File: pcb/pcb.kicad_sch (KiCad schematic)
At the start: 66 parts, among them IC1 W25Q16JVUXIQ, IC2 RP2040, IC3 AD8403ARUZ1-REEL, IC4 DS4432U+, IC5 XC6222D331MR-G, J1 USB_C_Receptacle, K1 G3VM-31WR_TR05_, Y2 ABM10AIG-12.000MHZ-2Z-T

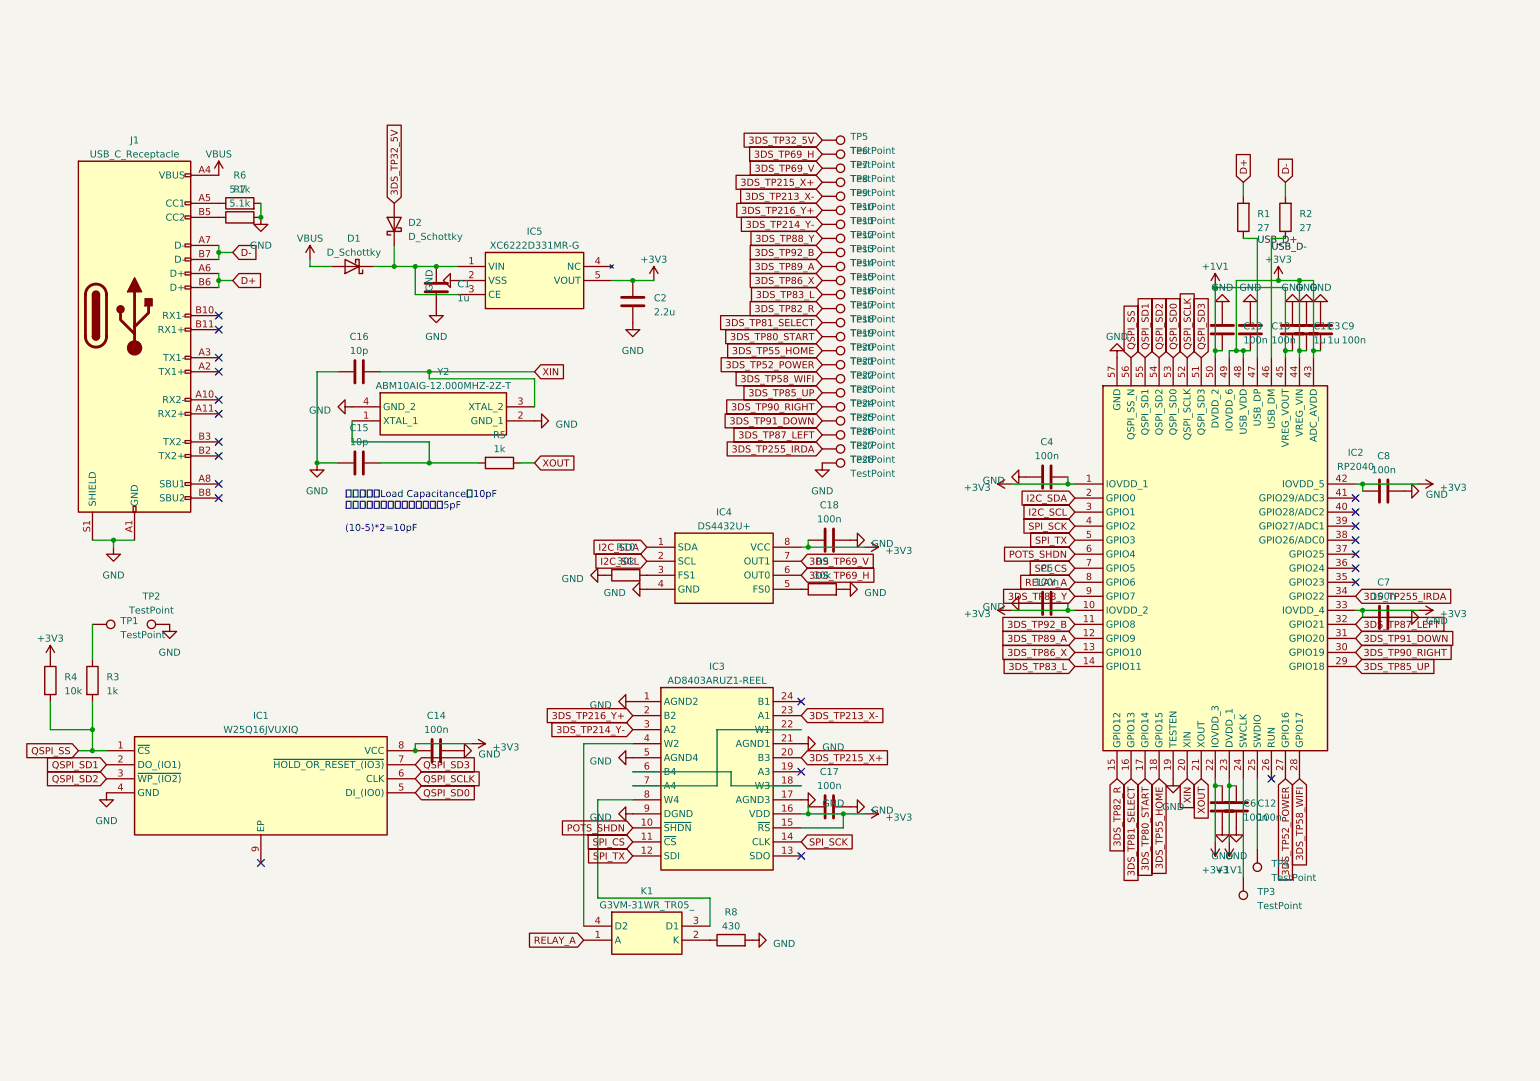
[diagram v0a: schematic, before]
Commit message: Update pcb
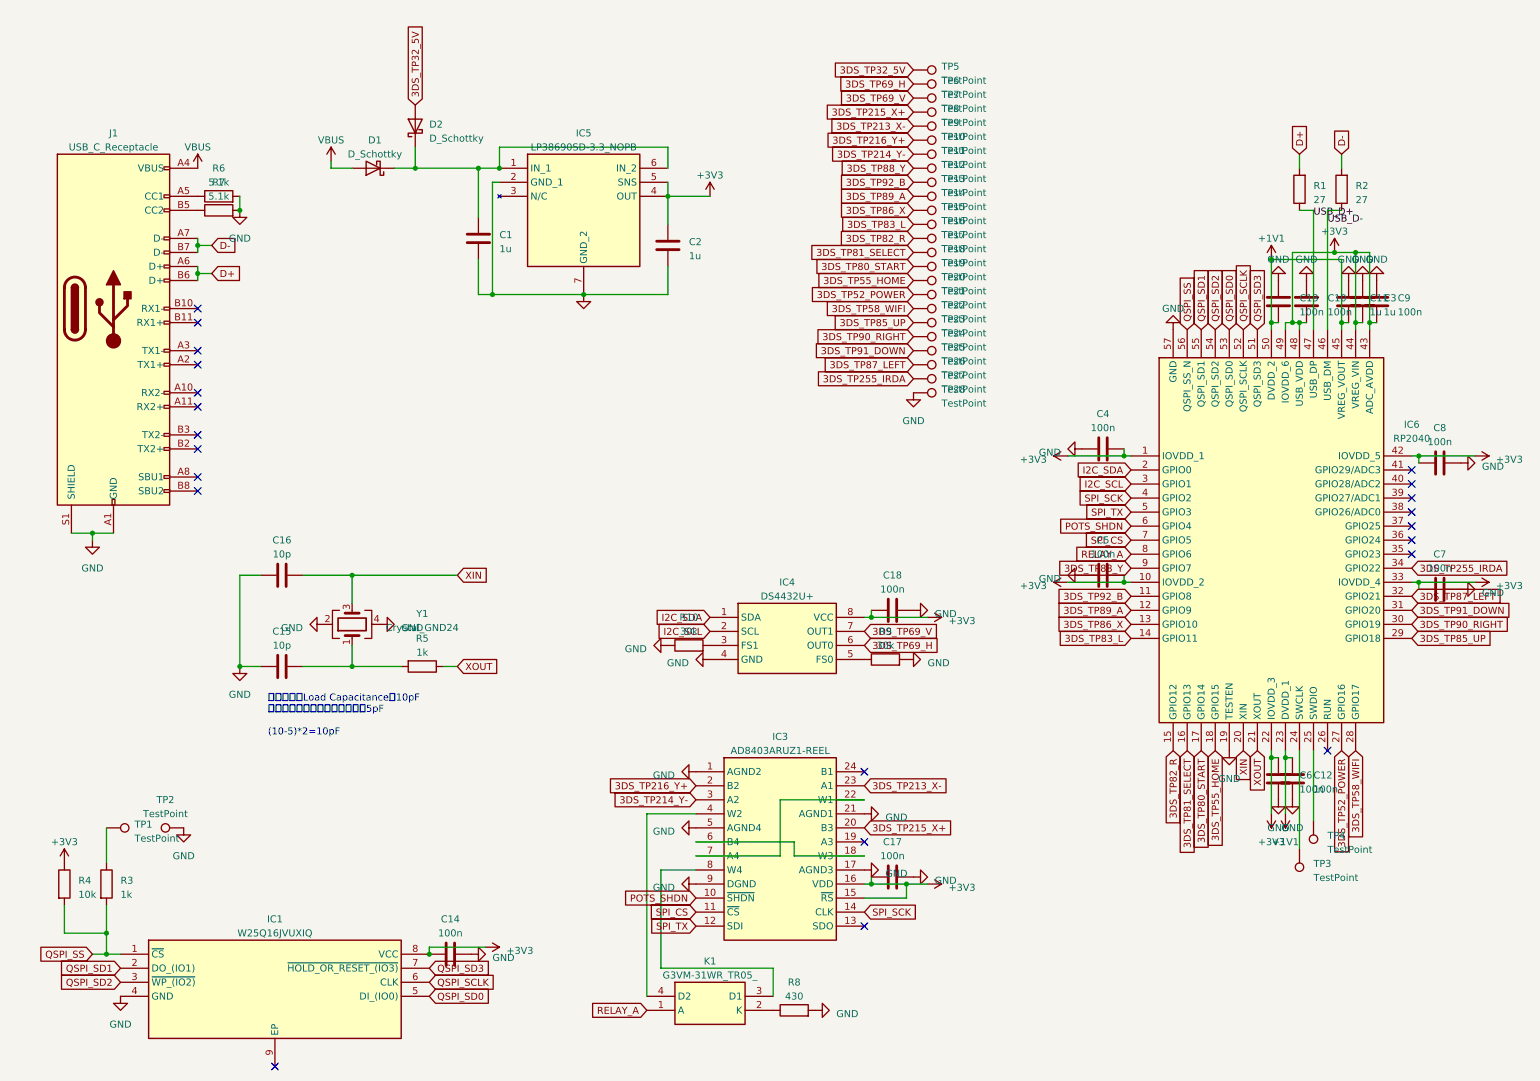
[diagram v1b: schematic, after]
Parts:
- removed IC2: RP2040, RP2040:QFN40P700X700X90-57N-D, symbol RP2040:RP2040
- removed IC5: XC6222D331MR-G, XC6222D331MR-G:SOT95P280X130-5N, symbol XC6222D331MR-G:XC6222D331MR-G
- removed Y2: ABM10AIG-12.000MHZ-2Z-T, ABM10AIG-12.000MHZ-2Z-T:ABM10AIG, symbol ABM10AIG-12_000MHZ-2Z-T:ABM10AIG-12.000MHZ-2Z-T
- added IC5: LP38690SD-3.3_NOPB, LP38690SD-3.3_NOPB:SON95P300X300X80-7N, symbol LP38690SD-3_3_NOPB:LP38690SD-3.3_NOPB
- added IC6: RP2040, RP2040:QFN40P700X700X90-57N-D, symbol RP2040:RP2040
- added Y1: Crystal_GND24, Crystal:Crystal_SMD_2520-4Pin_2.5x2.0mm, symbol Device:Crystal_GND24
- C1, C11, C3: footprint Capacitor_SMD:C_0201_0603Metric -> Capacitor_SMD:C_0402_1005Metric; LCSC C610030 -> C412453
- C10, C12, C13, C14, C17, C18, C4, C5, C6, C7, C8, C9: footprint Capacitor_SMD:C_0201_0603Metric -> Capacitor_SMD:C_0402_1005Metric; LCSC C5259862 -> C394158
- C15, C16: footprint Capacitor_SMD:C_0201_0603Metric -> Capacitor_SMD:C_0402_1005Metric; LCSC C396694 -> C161495
- C2: value 2.2u -> 1u; footprint Capacitor_SMD:C_0201_0603Metric -> Capacitor_SMD:C_0402_1005Metric; LCSC C5240383 -> C412453
- IC1: LCSC C2843335 -> (none)
- IC3: LCSC C652779 -> (none)
- IC4: LCSC C2679620 -> (none)
- R1, R2: footprint Resistor_SMD:R_0201_0603Metric -> Resistor_SMD:R_0402_1005Metric; LCSC C2484262 -> C102938
- R10, R9: footprint Resistor_SMD:R_0201_0603Metric -> Resistor_SMD:R_0402_1005Metric; LCSC C2991673 -> C144716
- R3, R5: footprint Resistor_SMD:R_0201_0603Metric -> Resistor_SMD:R_0402_1005Metric; LCSC C162776 -> C705665
- R4: footprint Resistor_SMD:R_0201_0603Metric -> Resistor_SMD:R_0402_1005Metric; LCSC C253350 -> C2991755
- R6, R7: footprint Resistor_SMD:R_0201_0603Metric -> Resistor_SMD:R_0402_1005Metric; LCSC C100142 -> C138073
- R8: footprint Resistor_SMD:R_0201_0603Metric -> Resistor_SMD:R_0402_1005Metric; LCSC C850675 -> C163462
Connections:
- net +1V1: now also IC6.23 (DVDD_1), IC6.45 (VREG_VOUT), IC6.50 (DVDD_2)
- net +3V3: now also IC5.4 (OUT), IC5.5 (SNS), IC6.1 (IOVDD_1), IC6.10 (IOVDD_2), IC6.22 (IOVDD_3), IC6.33 (IOVDD_4), IC6.42 (IOVDD_5), IC6.43 (ADC_AVDD), IC6.44 (VREG_VIN), IC6.48 (USB_VDD), IC6.49 (IOVDD_6)
- net 3DS_TP255_IRDA: now also IC6.34 (GPIO22)
- net 3DS_TP52_POWER: now also IC6.27 (GPIO16)
- net 3DS_TP55_HOME: now also IC6.18 (GPIO15)
- net 3DS_TP58_WIFI: now also IC6.28 (GPIO17)
- net 3DS_TP80_START: now also IC6.17 (GPIO14)
- net 3DS_TP81_SELECT: now also IC6.16 (GPIO13)
- net 3DS_TP82_R: now also IC6.15 (GPIO12)
- net 3DS_TP83_L: now also IC6.14 (GPIO11)
- net 3DS_TP85_UP: now also IC6.29 (GPIO18)
- net 3DS_TP86_X: now also IC6.13 (GPIO10)
- net 3DS_TP87_LEFT: now also IC6.32 (GPIO21)
- net 3DS_TP88_Y: now also IC6.9 (GPIO7)
- net 3DS_TP89_A: now also IC6.12 (GPIO9)
- net 3DS_TP90_RIGHT: now also IC6.30 (GPIO19)
- net 3DS_TP91_DOWN: now also IC6.31 (GPIO20)
- net 3DS_TP92_B: now also IC6.11 (GPIO8)
- net GND: now also IC5.2 (GND_1), IC5.7 (GND_2), IC6.19 (TESTEN), IC6.57 (GND), Y1.2, Y1.4
- net I2C_SCL: now also IC6.3 (GPIO1)
- net I2C_SDA: now also IC6.2 (GPIO0)
- net POTS_SHDN: now also IC6.6 (GPIO4)
- net QSPI_SCLK: now also IC6.52 (QSPI_SCLK)
- net QSPI_SD0: now also IC6.53 (QSPI_SD0)
- net QSPI_SD1: now also IC6.55 (QSPI_SD1)
- net QSPI_SD2: now also IC6.54 (QSPI_SD2)
- net QSPI_SD3: now also IC6.51 (QSPI_SD3)
- net QSPI_SS: now also IC6.56 (QSPI_SS_N)
- net RELAY_A: now also IC6.8 (GPIO6)
- net SPI_CS: now also IC6.7 (GPIO5)
- net SPI_SCK: now also IC6.4 (GPIO2)
- net SPI_TX: now also IC6.5 (GPIO3)
- net USB_D+: now also IC6.47 (USB_DP)
- net USB_D-: now also IC6.46 (USB_DM)
- net XIN: now also IC6.20 (XIN), Y1.3
- net XOUT: now also IC6.21 (XOUT)
- net at C1.1, D1.1 (K), D2.1 (K): now also IC5.1 (IN_1), IC5.6 (IN_2)
- net at C15.1, R5.2: now also Y1.1
- net at TP4.1: now also IC6.25 (SWDIO)
- net at TP3.1: now also IC6.24 (SWCLK)
